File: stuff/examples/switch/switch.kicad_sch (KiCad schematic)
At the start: 4 parts

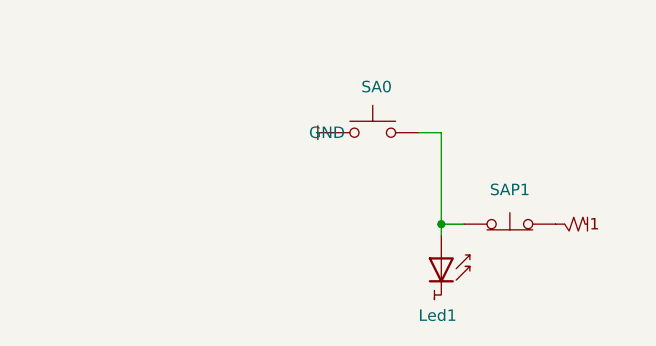
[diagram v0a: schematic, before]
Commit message: pre V2 commit
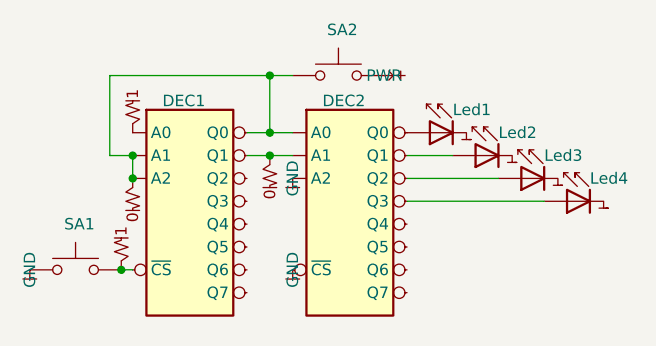
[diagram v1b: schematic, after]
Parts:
- removed SA0: SW_Push, symbol Switch:SW_Push
- removed SAP1: SW_Push_Open, symbol Switch:SW_Push_Open
- added DEC1, DEC2: decode_3_bit, symbol chip:DECODE_3BIT
- added Led2, Led3, Led4: ~, symbol chip:LED
- added SA1, SA2: SW_Push, symbol Switch:SW_Push
- added pulldown1, pulldown2: pull_down, symbol chip:PULLDOWN
- added pullup2: pull_up, symbol chip:PULLUP
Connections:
- net gnd: now also DEC2.12 (~{CS}), DEC2.3 (A2), SA1.1
- net at Led1.1 (IN): now also DEC2.4 (Q0)
- net at pullup1.1 (OUT): now also DEC1.1 (A0)
- new net: DEC2.5 (Q1), Led2.1 (IN)
- new net: DEC1.2 (A1), DEC1.3 (A2), DEC1.4 (Q0), DEC2.1 (A0), SA2.1, pulldown1.1 (OUT)
- new net: DEC1.12 (~{CS}), SA1.2, pullup2.1 (OUT)
- new net: DEC1.5 (Q1), DEC2.2 (A1), pulldown2.1 (OUT)
- new net: DEC2.6 (Q2), Led3.1 (IN)
- new net: DEC2.7 (Q3), Led4.1 (IN)
- new net pwr: SA2.2
